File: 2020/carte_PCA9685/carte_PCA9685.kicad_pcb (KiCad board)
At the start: 2 copper layers, 33 parts, among them J1 Screw_Terminal_01x02, J10 Conn_01x02, J11 Servo_1, J12 Servo_2, J13 Servo_3, J14 Servo_4, J15 Servo_5, J16 Servo_6, J17 Servo_10, J18 Conn_01x02, J2 i2c, J3 Conn_01x02, J4 Conn_01x02, J5 Conn_01x02, J6 Conn_01x02, J7 Servo_7, J8 Servo_8, J9 Servo_9, U1 LM2596_module, U2 IRLML6344, U3 IRLML6344, U4 PCA9685PW, U5 IRLML6344, U6 IRLML6344, U7 IRLML6344, U8 IRLML6344

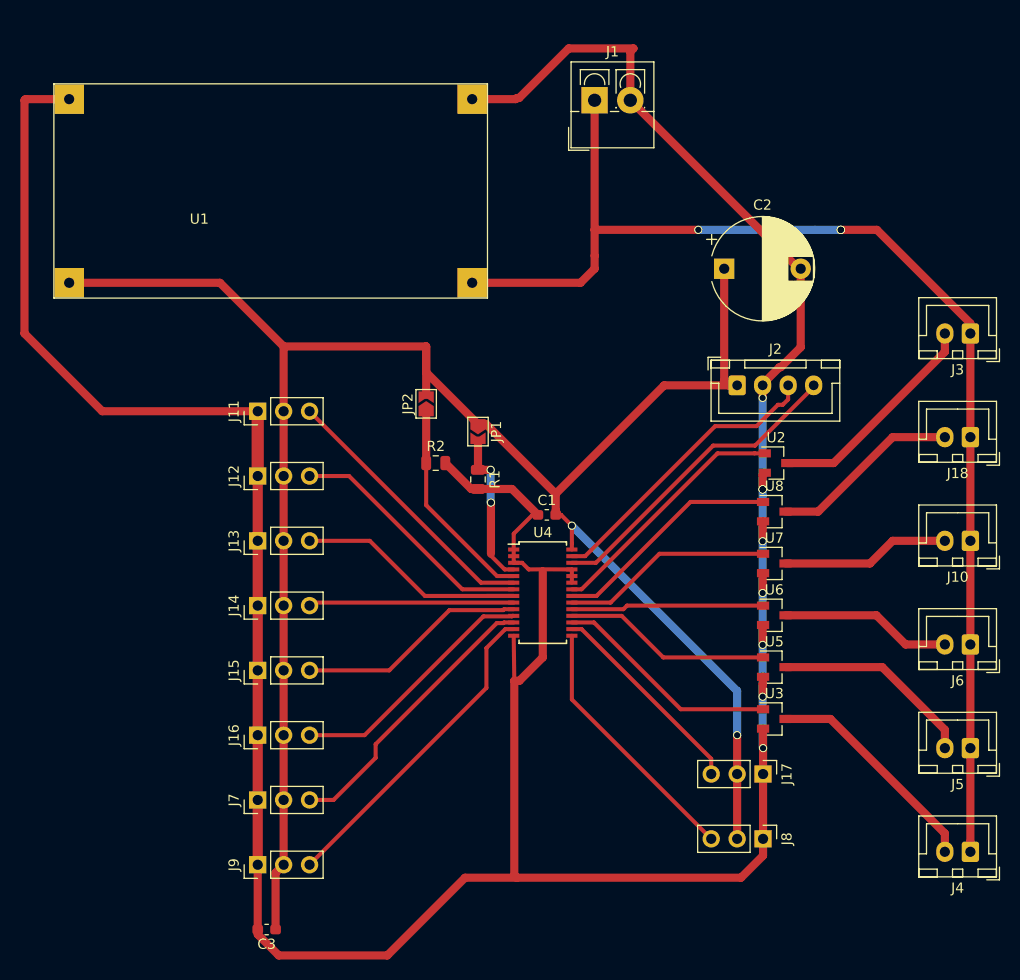
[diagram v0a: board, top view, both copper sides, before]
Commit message: Fin carte elec 2020 robot-a
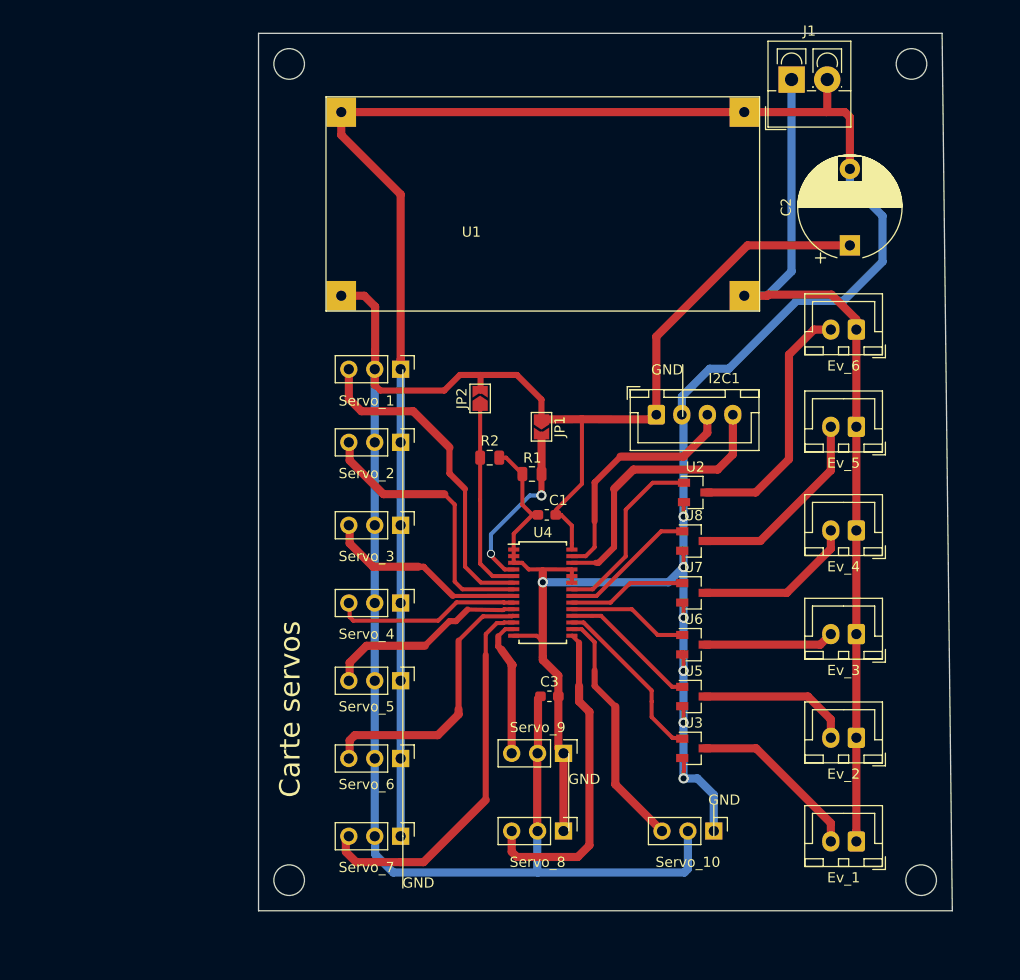
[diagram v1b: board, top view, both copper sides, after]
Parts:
- removed J11: Servo_1, Connector_PinHeader_2.54mm:PinHeader_1x03_P2.54mm_Vertical
- removed J12: Servo_2, Connector_PinHeader_2.54mm:PinHeader_1x03_P2.54mm_Vertical
- removed J13: Servo_3, Connector_PinHeader_2.54mm:PinHeader_1x03_P2.54mm_Vertical
- removed J14: Servo_4, Connector_PinHeader_2.54mm:PinHeader_1x03_P2.54mm_Vertical
- removed J15: Servo_5, Connector_PinHeader_2.54mm:PinHeader_1x03_P2.54mm_Vertical
- removed J16: Servo_6, Connector_PinHeader_2.54mm:PinHeader_1x03_P2.54mm_Vertical
- removed J17: Servo_10, Connector_PinHeader_2.54mm:PinHeader_1x03_P2.54mm_Vertical
- removed J7: Servo_7, Connector_PinHeader_2.54mm:PinHeader_1x03_P2.54mm_Vertical
- removed J8: Servo_8, Connector_PinHeader_2.54mm:PinHeader_1x03_P2.54mm_Vertical
- removed J9: Servo_9, Connector_PinHeader_2.54mm:PinHeader_1x03_P2.54mm_Vertical
- added  : MountingHole_3mm, MountingHole:MountingHole_3mm, F.Cu at (125.0, 112.0)
- added  : MountingHole_3mm, MountingHole:MountingHole_3mm, F.Cu at (186.9, 112.0)
- added  : MountingHole_3mm, MountingHole:MountingHole_3mm, F.Cu at (186.0, 32.0)
- added  : MountingHole_3mm, MountingHole:MountingHole_3mm, F.Cu at (125.0, 32.0)
- added G***: LOGO, myFootprints:logo_enac_robotique, B.Cu at (152.9, 62.0)
- added Servo_1: Conn_01x03, Connector_PinHeader_2.54mm:PinHeader_1x03_P2.54mm_Vertical, F.Cu at (135.9, 61.9)
- added Servo_10: Conn_01x03, Connector_PinHeader_2.54mm:PinHeader_1x03_P2.54mm_Vertical, F.Cu at (166.6, 107.2)
- added Servo_2: Conn_01x03, Connector_PinHeader_2.54mm:PinHeader_1x03_P2.54mm_Vertical, F.Cu at (135.9, 69.1)
- added Servo_3: Conn_01x03, Connector_PinHeader_2.54mm:PinHeader_1x03_P2.54mm_Vertical, F.Cu at (135.9, 77.2)
- added Servo_4: Conn_01x03, Connector_PinHeader_2.54mm:PinHeader_1x03_P2.54mm_Vertical, F.Cu at (135.9, 84.8)
- added Servo_5: Conn_01x03, Connector_PinHeader_2.54mm:PinHeader_1x03_P2.54mm_Vertical, F.Cu at (135.9, 92.5)
- added Servo_6: Conn_01x03, Connector_PinHeader_2.54mm:PinHeader_1x03_P2.54mm_Vertical, F.Cu at (135.9, 100.1)
- added Servo_7: Conn_01x03, Connector_PinHeader_2.54mm:PinHeader_1x03_P2.54mm_Vertical, F.Cu at (135.9, 107.7)
- added Servo_8: Conn_01x03, Connector_PinHeader_2.54mm:PinHeader_1x03_P2.54mm_Vertical, F.Cu at (151.9, 107.2)
- added Servo_9: Conn_01x03, Connector_PinHeader_2.54mm:PinHeader_1x03_P2.54mm_Vertical, F.Cu at (151.9, 99.6)
- I2C1: renamed from J2; value i2c -> Conn_01x04
- moved C3 35.9 mm to (150.5, 94.0), turned to 0 degrees
- moved U1 26.7 mm to (149.9, 45.7)
- moved J1 19.4 mm to (174.2, 33.5)
- moved C2 12.5 mm to (180.0, 49.8), turned to 90 degrees
- moved Ev_1 11.2 mm to (180.6, 108.2)
- moved Ev_2 11.2 mm to (180.6, 98.0)
- moved Ev_3 11.2 mm to (180.6, 87.9)
- moved Ev_5 11.2 mm to (180.6, 67.6)
- moved Ev_4 11.2 mm to (180.6, 77.7)
- moved Ev_6 11.2 mm to (180.6, 58.0)
- moved U7 8.43 mm to (164.6, 83.8)
- moved U8 8.43 mm to (164.6, 78.8)
- moved U3 8.43 mm to (164.6, 99.1)
- moved U5 8.43 mm to (164.6, 94.0)
- moved U6 8.43 mm to (164.6, 88.9)
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- renumbered J4 to Ev_1, J5 to Ev_2, J6 to Ev_3, J10 to Ev_4, J18 to Ev_5, J3 to Ev_6
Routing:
- net GND: track 336.9 -> 286.7 mm, vias 8 -> 7
- net +12V: track 121.5 -> 88.3 mm, vias 3 -> 0
- net /PWM_servo_9: track 31.9 -> 13.8 mm
- net /PWM_servo_7: track 28.0 -> 37.8 mm
- net /ev_5: track 22.6 -> 13.4 mm
- net /ev_4: track 20.7 -> 11.6 mm
- net +5V: track 198.4 -> 189.5 mm, vias 2 -> 0
- net /ev_3: track 18.9 -> 11.9 mm
- net /ev_2: track 20.4 -> 13.7 mm
- net /ev_6: track 24.4 -> 18.0 mm
- net /PWM_servo_8: track 25.6 -> 31.6 mm
- net /PWM_servo_1: track 27.0 -> 32.4 mm
- net /ev_1: track 22.3 -> 17.0 mm
- net Net-(Ev_1-Pad2): track 22.1 -> 17.2 mm
- net Net-(Ev_2-Pad2): track 20.0 -> 15.1 mm
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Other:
- board outline added: 68 x 86 mm
- board text added: "Antoine @ ENAC 2020"
- board text added: "Carte servos"
- board text added: "GND"
